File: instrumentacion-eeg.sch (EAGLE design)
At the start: 39 parts, among them IC1 LMV321AIDCKR, IC15 LMV321AIDCKR, IC16 LMV321AIDCKR, IC2 ESP32-S3-WROOM-1-N4R2, IC3 LMV321AIDCKR, IC5 MCP73831T-2ACI_OT, IC7 AD8226ARZ, IC9 LP38692MP-3.3_NOPB, J1 USB3500-30-A-KIT, J3 SJ-3523-SMT-TR, J4 1769

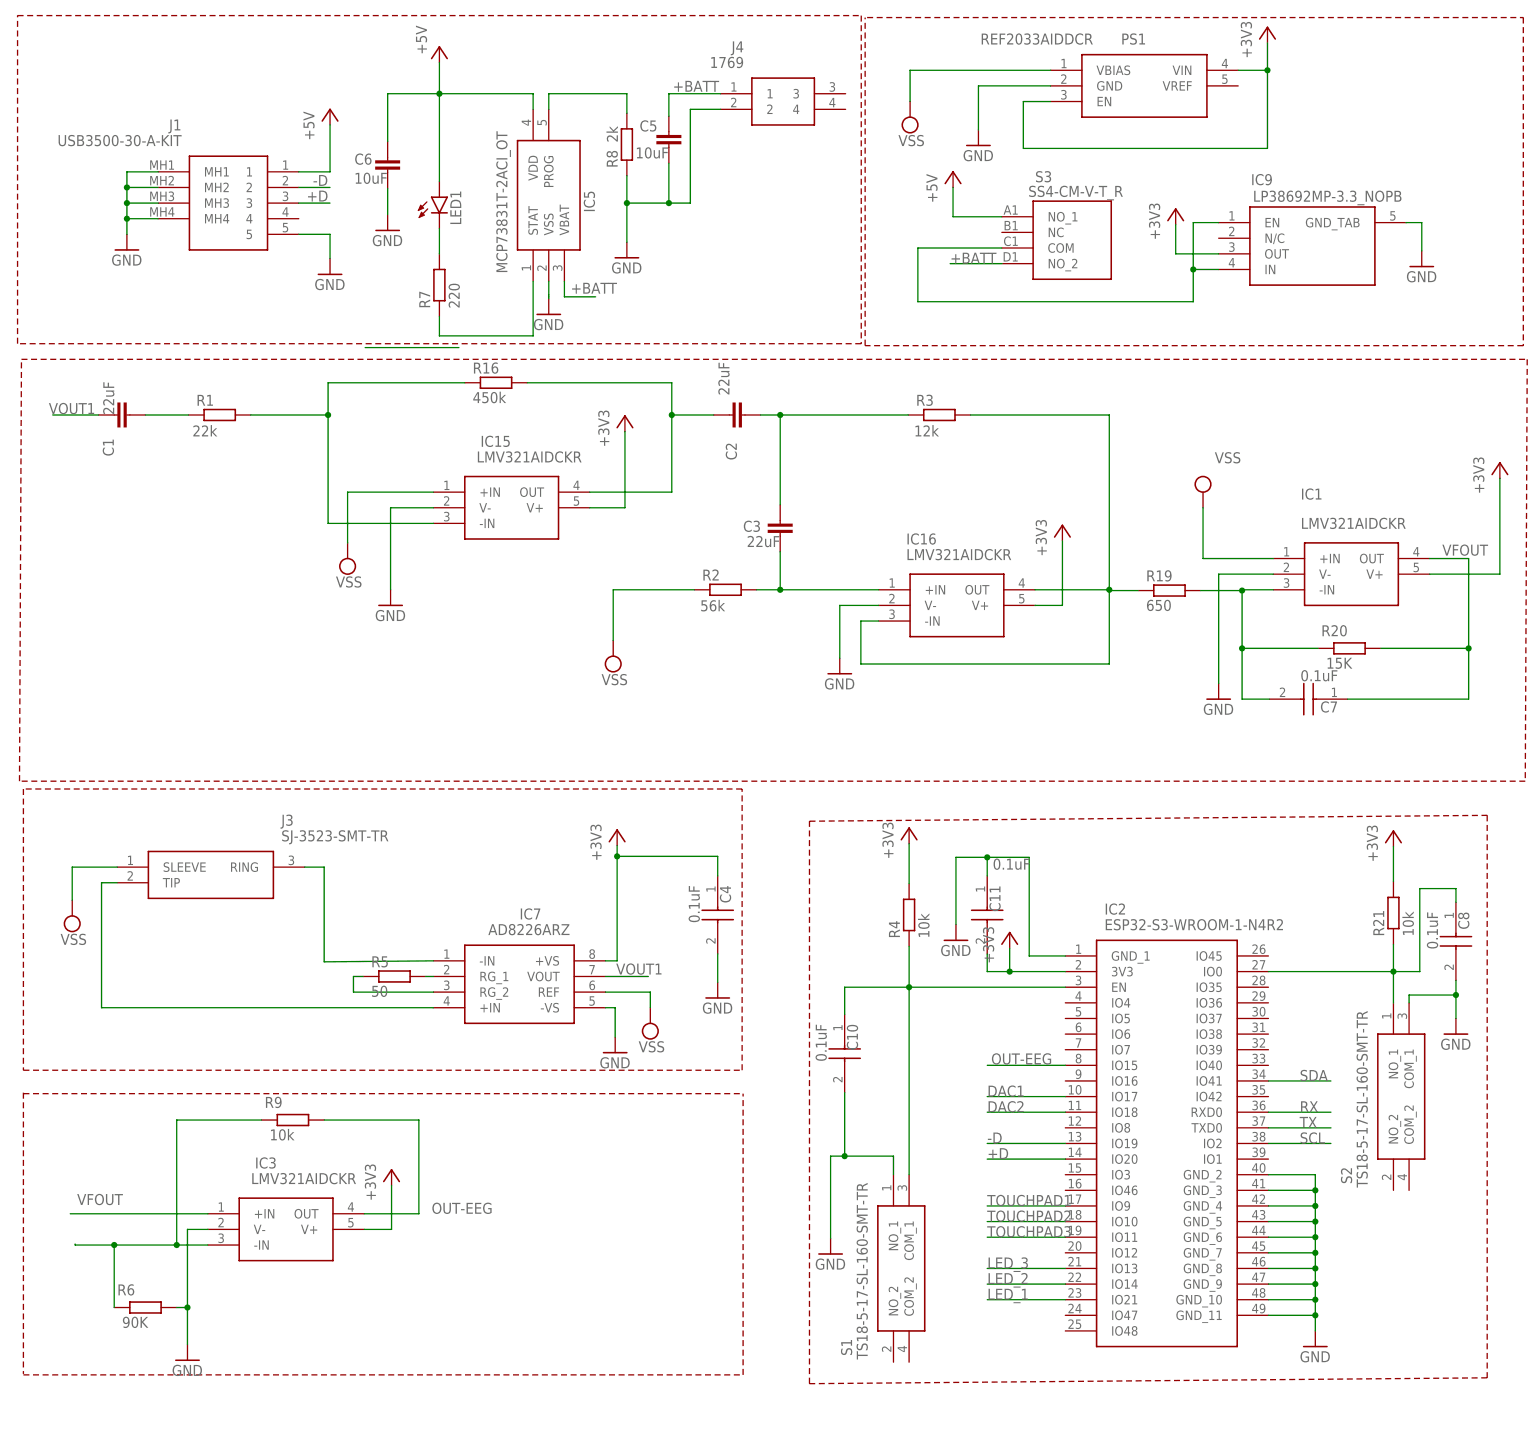
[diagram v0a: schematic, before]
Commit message: Agrego archivos
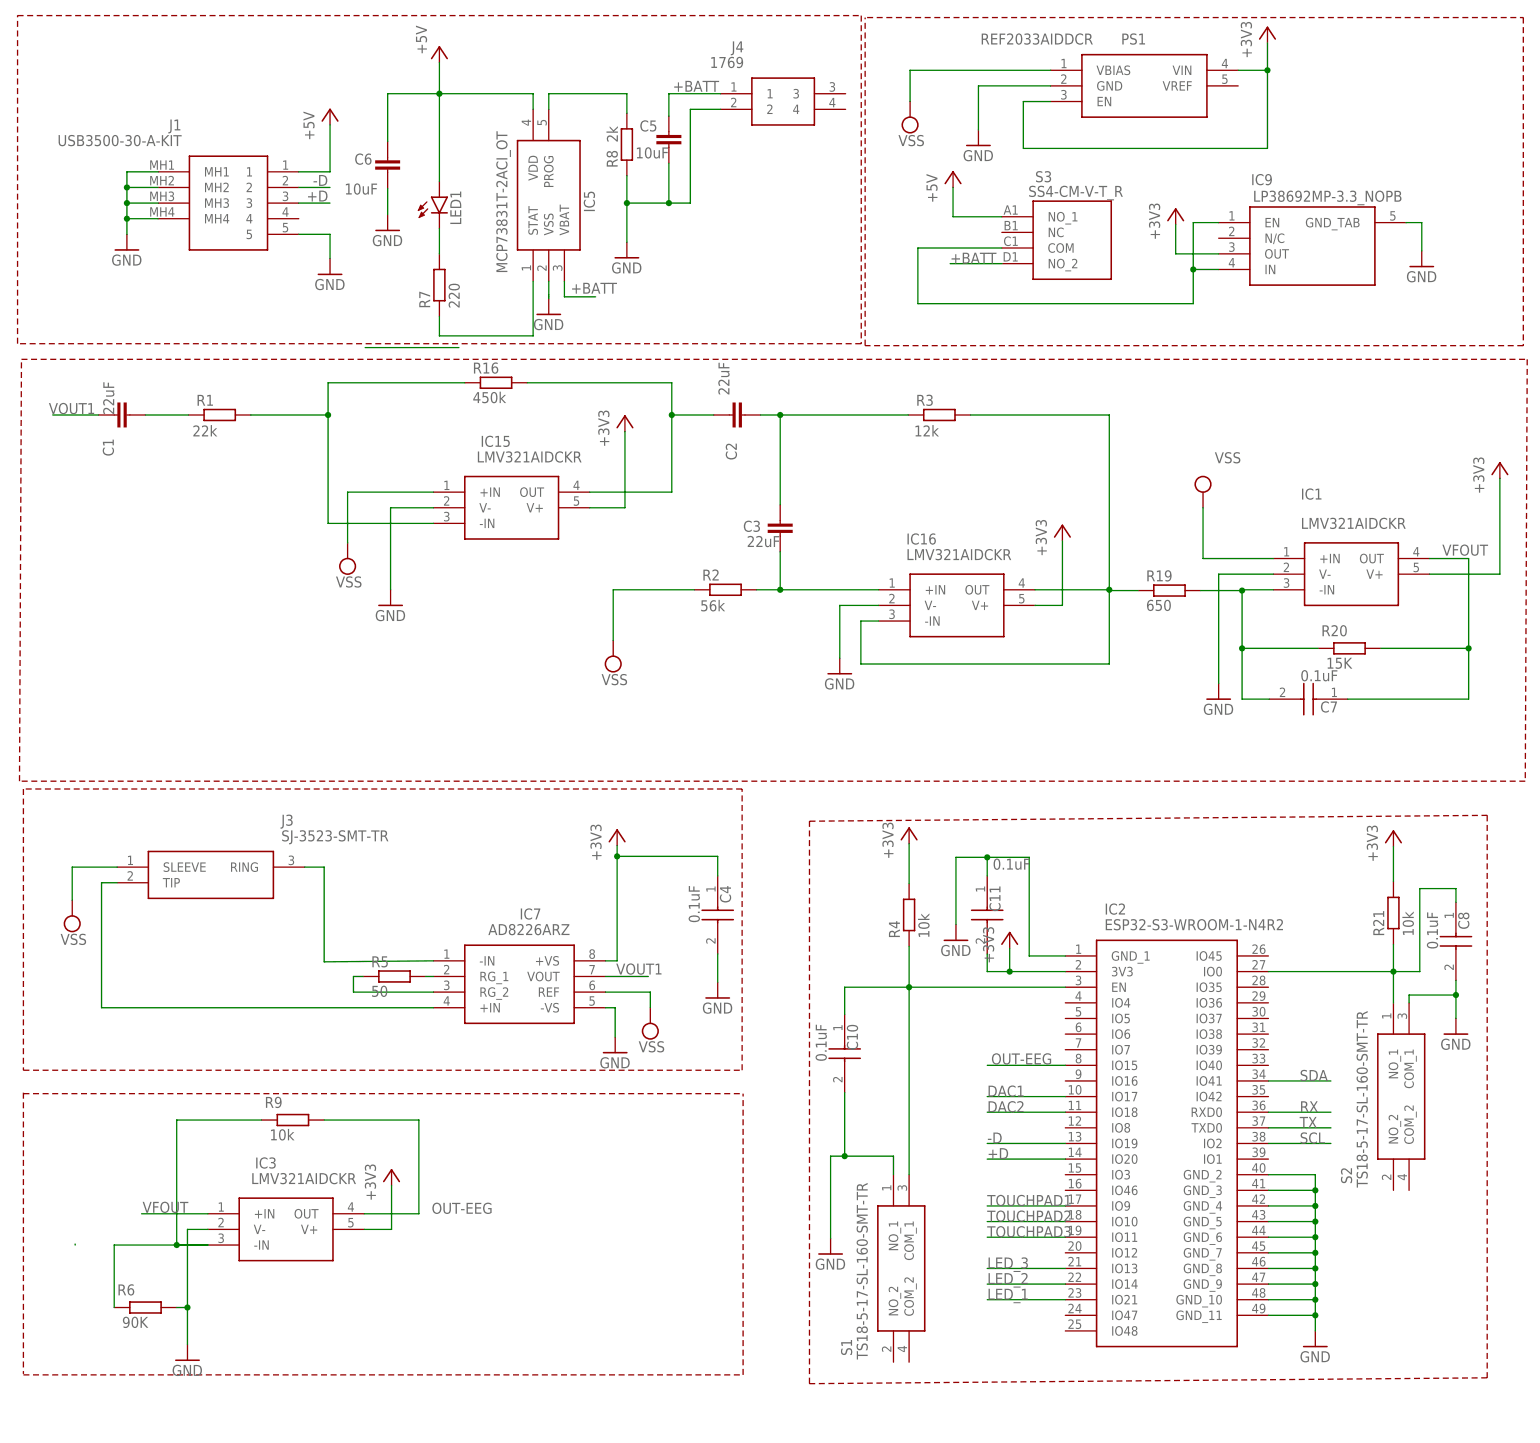
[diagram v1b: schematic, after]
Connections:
- removed net N$15: IC3.+IN
- removed net N$7: R6.1
- net N$14: now also R6.1
- net VFOUT: now also IC3.+IN
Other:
- note removed: "VFOUT"
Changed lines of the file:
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@@
 <wire x1="114.45875" y1="-107.95" x2="114.45875" y2="-62.23" width="0.1524" layer="94" style="shortdash"/>
 <wire x1="-2.54" y1="-107.95" x2="114.3" y2="-107.95" width="0.1524" layer="94" style="shortdash"/>
-<text x="6.19125" y="-80.3275" size="1.778" layer="95">VFOUT</text>
 </plain>
 <instances>
@@
 <attribute name="NAME" x="54.19725" y="90.58275" size="1.778" layer="95" rot="R180"/>
 <attribute name="VALUE" x="55.14975" y="92.17025" size="1.778" layer="96" rot="R180"/>
-<attribute name="POPULARITY" x="56.67375" y="87.47125" size="1.778" layer="96" rot="R180"/>
+<attribute name="POPULARITY" x="55.08625" y="85.725" size="1.778" layer="96" rot="R180"/>
 </instance>
 <instance part="C5" gate="G$1" x="102.39375" y="91.59875" smashed="yes" rot="R180">
@@
 <wire x1="187.6425" y1="79.375" x2="187.6425" y2="71.755" width="0.1524" layer="91"/>
 <pinref part="IC9" gate="G$1" pin="EN"/>
-<wire x1="187.6425" y1="71.755" x2="187.6425" y2="66.51625" width="0.1524" layer="91"/>
+<wire x1="187.6425" y1="71.755" x2="187.6425" y2="66.19875" width="0.1524" layer="91"/>
 <wire x1="187.6425" y1="79.375" x2="191.77" y2="79.375" width="0.1524" layer="91"/>
 <pinref part="S3" gate="G$1" pin="COM"/>
 <wire x1="156.5275" y1="75.2475" x2="142.875" y2="75.2475" width="0.1524" layer="91"/>
-<wire x1="142.875" y1="75.2475" x2="142.875" y2="66.51625" width="0.1524" layer="91"/>
-<wire x1="142.875" y1="66.51625" x2="187.6425" y2="66.51625" width="0.1524" layer="91"/>
+<wire x1="142.875" y1="75.2475" x2="142.875" y2="66.19875" width="0.1524" layer="91"/>
+<wire x1="142.875" y1="66.19875" x2="187.6425" y2="66.19875" width="0.1524" layer="91"/>
 <pinref part="IC9" gate="G$1" pin="IN"/>
 <wire x1="191.77" y1="71.755" x2="187.6425" y2="71.755" width="0.1524" layer="91"/>
@@
 <label x="228.12375" y="25.24125" size="1.778" layer="95"/>
 </segment>
+<segment>
+<pinref part="IC3" gate="G$1" pin="+IN"/>
+<wire x1="27.46375" y1="-81.75625" x2="16.66875" y2="-81.75625" width="0.1524" layer="91"/>
+<label x="16.8275" y="-81.5975" size="1.778" layer="95"/>
+</segment>
 </net>
 <net name="N$2" class="0">
@@
 </segment>
 </net>
-<net name="N$7" class="0">
-<segment>
-<pinref part="R6" gate="G$1" pin="1"/>
-<wire x1="12.22375" y1="-96.99625" x2="12.22375" y2="-86.83625" width="0.1524" layer="91"/>
-<junction x="12.22375" y="-86.83625"/>
-</segment>
-</net>
 <net name="N$14" class="0">
 <segment>
+<pinref part="R9" gate="G$1" pin="1"/>
 <wire x1="22.38375" y1="-86.83625" x2="22.38375" y2="-66.51625" width="0.1524" layer="91"/>
-<pinref part="R9" gate="G$1" pin="1"/>
 <wire x1="22.38375" y1="-66.51625" x2="36.195" y2="-66.51625" width="0.1524" layer="91"/>
 <pinref part="IC3" gate="G$1" pin="-IN"/>
 <wire x1="27.46375" y1="-86.83625" x2="22.38375" y2="-86.83625" width="0.1524" layer="91"/>
-<wire x1="22.38375" y1="-86.83625" x2="5.87375" y2="-86.83625" width="0.1524" layer="91"/>
-<wire x1="5.87375" y1="-86.83625" x2="5.87375" y2="-86.6775" width="0.1524" layer="91"/>
+<pinref part="R6" gate="G$1" pin="1"/>
+<wire x1="12.22375" y1="-96.99625" x2="12.22375" y2="-86.83625" width="0.1524" layer="91"/>
+<wire x1="12.22375" y1="-86.83625" x2="22.38375" y2="-86.83625" width="0.1524" layer="91"/>
 <junction x="22.38375" y="-86.83625"/>
-</segment>
-</net>
-<net name="N$15" class="0">
-<segment>
-<pinref part="IC3" gate="G$1" pin="+IN"/>
-<wire x1="27.46375" y1="-81.75625" x2="5.08" y2="-81.75625" width="0.1524" layer="91"/>
+<wire x1="22.38375" y1="-86.83625" x2="27.46375" y2="-86.83625" width="0.1524" layer="91"/>
 </segment>
 </net>
@@
 </segment>
 </net>
+<net name="N$8" class="0">
+<segment>
+<wire x1="5.87375" y1="-86.83625" x2="5.87375" y2="-86.6775" width="0.1524" layer="91"/>
+</segment>
+</net>
